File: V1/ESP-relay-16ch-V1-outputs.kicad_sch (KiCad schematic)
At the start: 40 parts

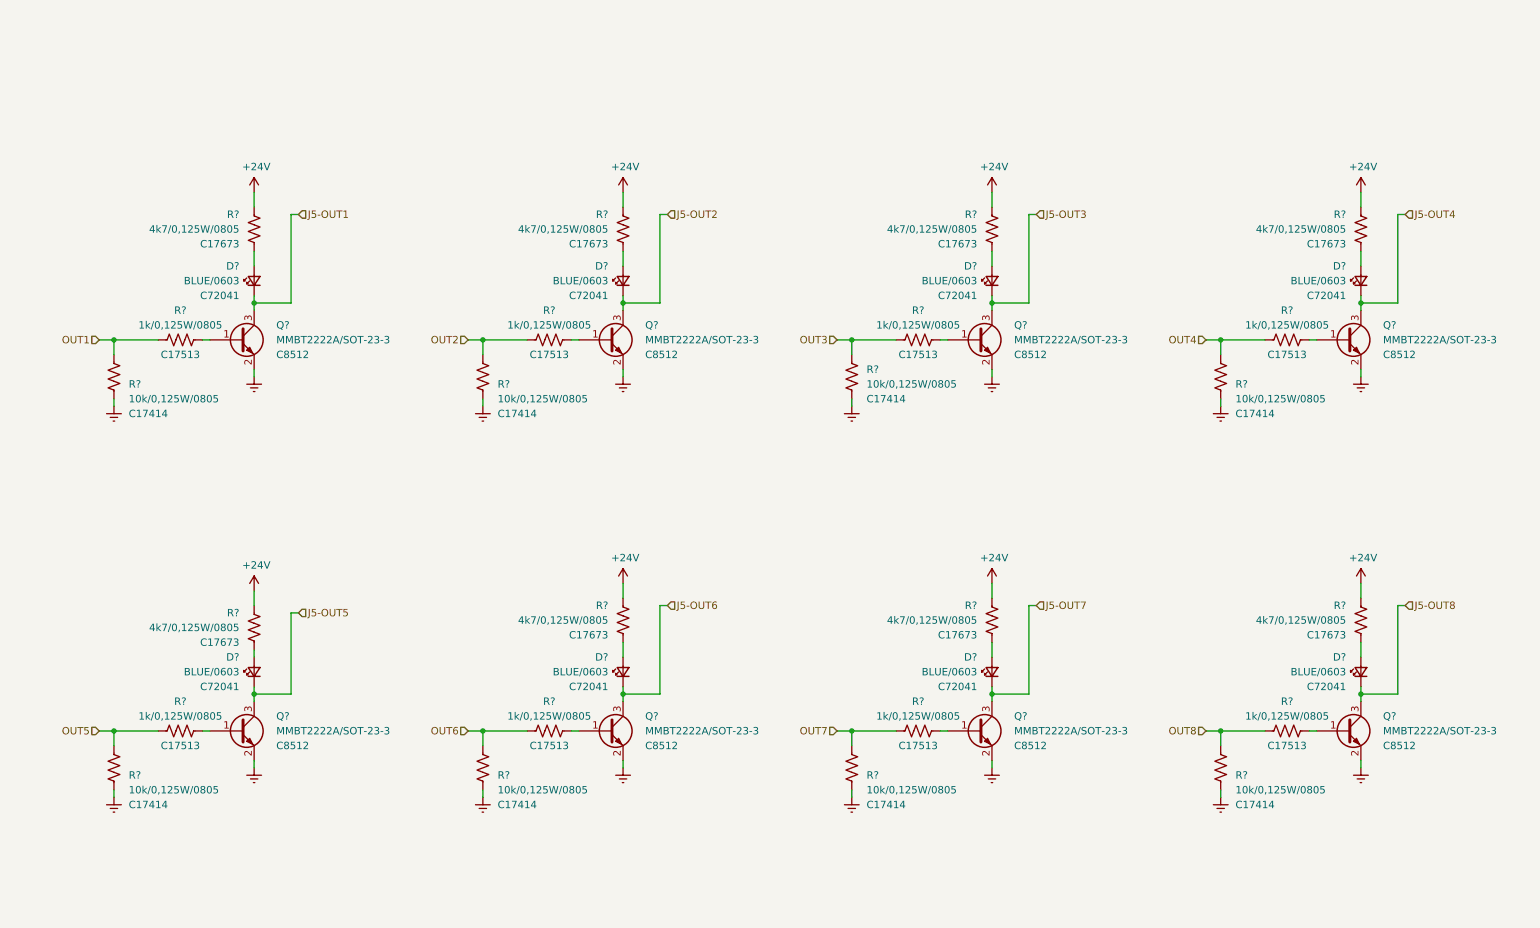
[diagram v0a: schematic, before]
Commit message: Dev updates
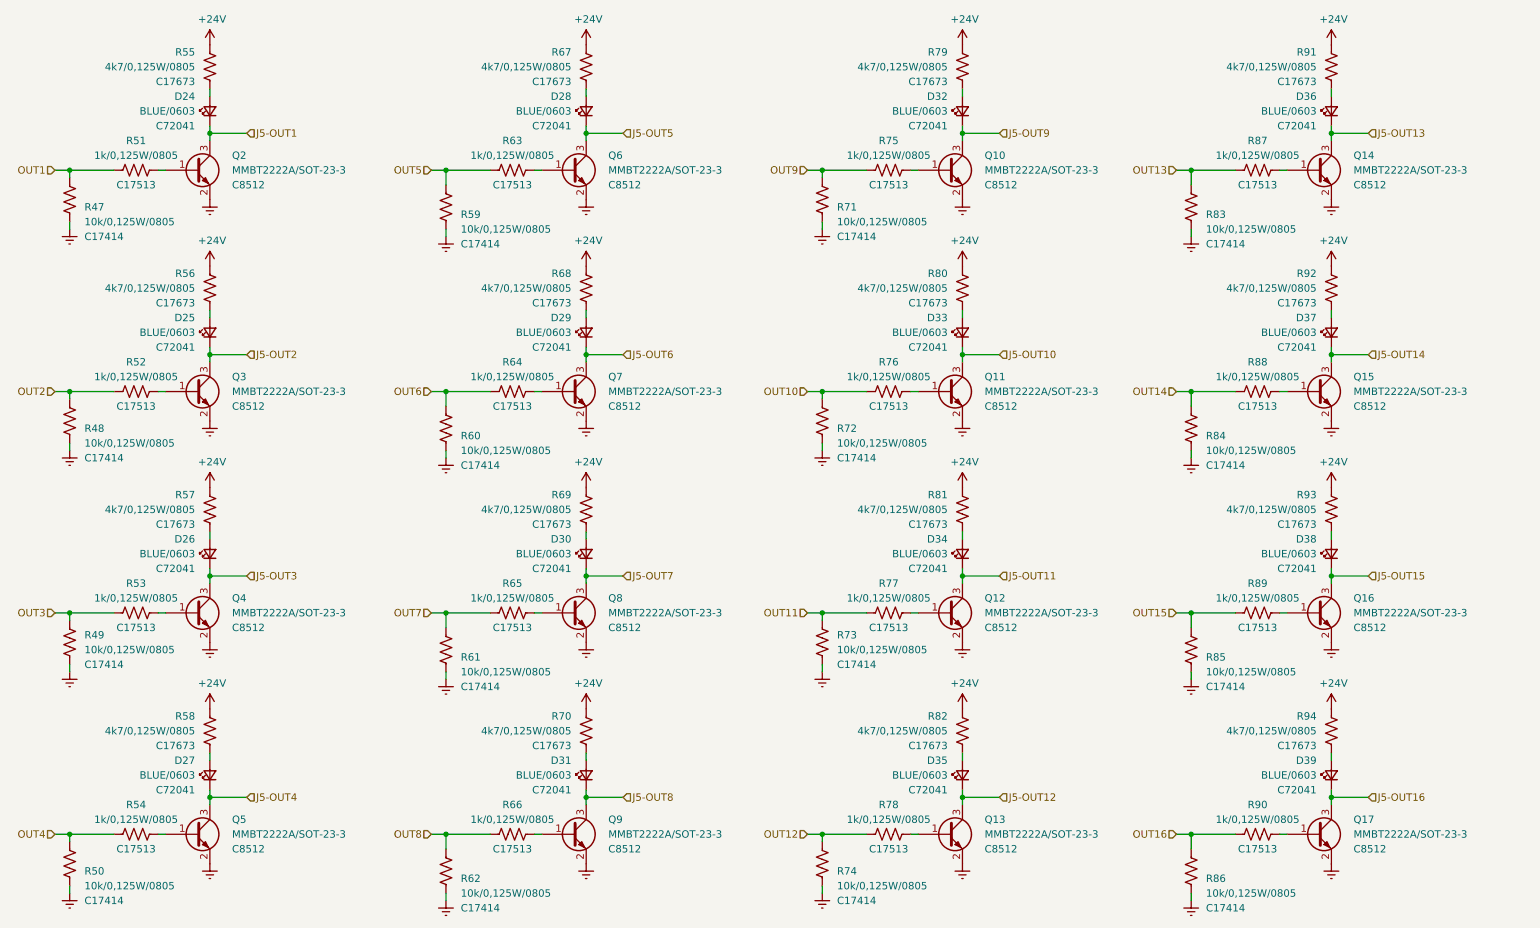
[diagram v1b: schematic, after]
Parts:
- added D32, D33, D34, D35, D36, D37, D38, D39: BLUE/0603, Tales:LED_0603_1608Metric, symbol Device:LED_Small
- added Q10, Q11, Q12, Q13, Q14, Q15, Q16, Q17: MMBT2222A/SOT-23-3, Tales:SOT-23, symbol Device:Q_NPN_BEC
- added R71, R72, R73, R74, R83, R84, R85, R86: 10k/0,125W/0805, Tales:R_0805_2012Metric, symbol Device:R_US
- added R75, R76, R77, R78, R87, R88, R89, R90: 1k/0,125W/0805, Tales:R_0805_2012Metric, symbol Device:R_US
- added R79, R80, R81, R82, R91, R92, R93, R94: 4k7/0,125W/0805, Tales:R_0805_2012Metric, symbol Device:R_US
- gave numbers to parts that had none: 40
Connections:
- net +24V: now also R79.1, R80.1, R81.1, R82.1, R91.1, R92.1, R93.1, R94.1
- net GNDREF: now also Q10.2 (E), Q11.2 (E), Q12.2 (E), Q13.2 (E), Q14.2 (E), Q15.2 (E), Q16.2 (E), Q17.2 (E), R71.2, R72.2, R73.2, R74.2, R83.2, R84.2, R85.2, R86.2
- new net: D37.2 (A), R92.2
- new net: Q10.1 (B), R75.1
- new net: Q17.1 (B), R90.1
- new net: D39.2 (A), R94.2
- new net: Q15.1 (B), R88.1
- new net: Q12.1 (B), R77.1
- new net: D35.2 (A), R82.2
- new net: Q14.1 (B), R87.1
- new net: D33.2 (A), R80.2
- new net: D34.2 (A), R81.2
- new net: D38.2 (A), R93.2
- new net: Q11.1 (B), R76.1
- new net: D36.2 (A), R91.2
- new net: Q13.1 (B), R78.1
- new net: Q16.1 (B), R89.1
- new net: D32.2 (A), R79.2
- new net J5-OUT10: D33.1 (K), Q11.3 (C)
- new net J5-OUT11: D34.1 (K), Q12.3 (C)
- new net J5-OUT12: D35.1 (K), Q13.3 (C)
- new net J5-OUT13: D36.1 (K), Q14.3 (C)
- new net J5-OUT14: D37.1 (K), Q15.3 (C)
- new net J5-OUT15: D38.1 (K), Q16.3 (C)
- new net J5-OUT16: D39.1 (K), Q17.3 (C)
- new net J5-OUT9: D32.1 (K), Q10.3 (C)
- new net OUT10: R72.1, R76.2
- new net OUT11: R73.1, R77.2
- new net OUT12: R74.1, R78.2
- new net OUT13: R83.1, R87.2
- new net OUT14: R84.1, R88.2
- new net OUT15: R85.1, R89.2
- new net OUT16: R86.1, R90.2
- new net OUT9: R71.1, R75.2
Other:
- moved on the sheet: D24, D25, D26, D27, D28, D29, D30, D31, Q2, Q3, Q4, Q5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
